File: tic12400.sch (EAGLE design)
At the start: 14 parts, among them X1 22-23-2031

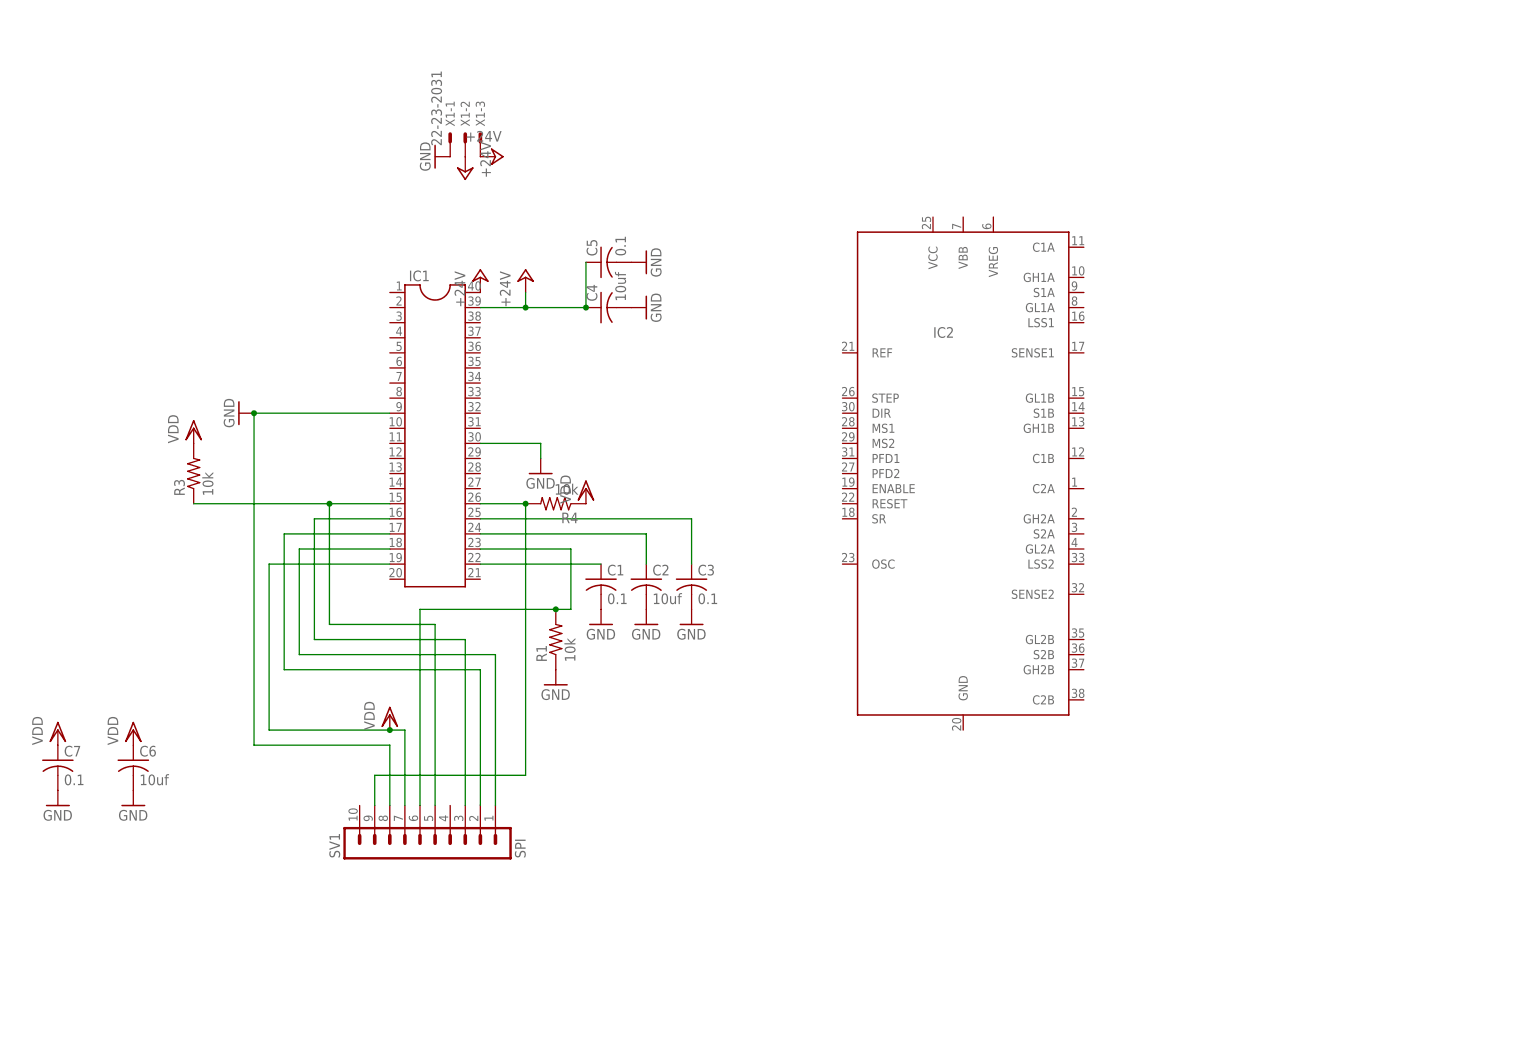
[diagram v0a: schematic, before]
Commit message: up
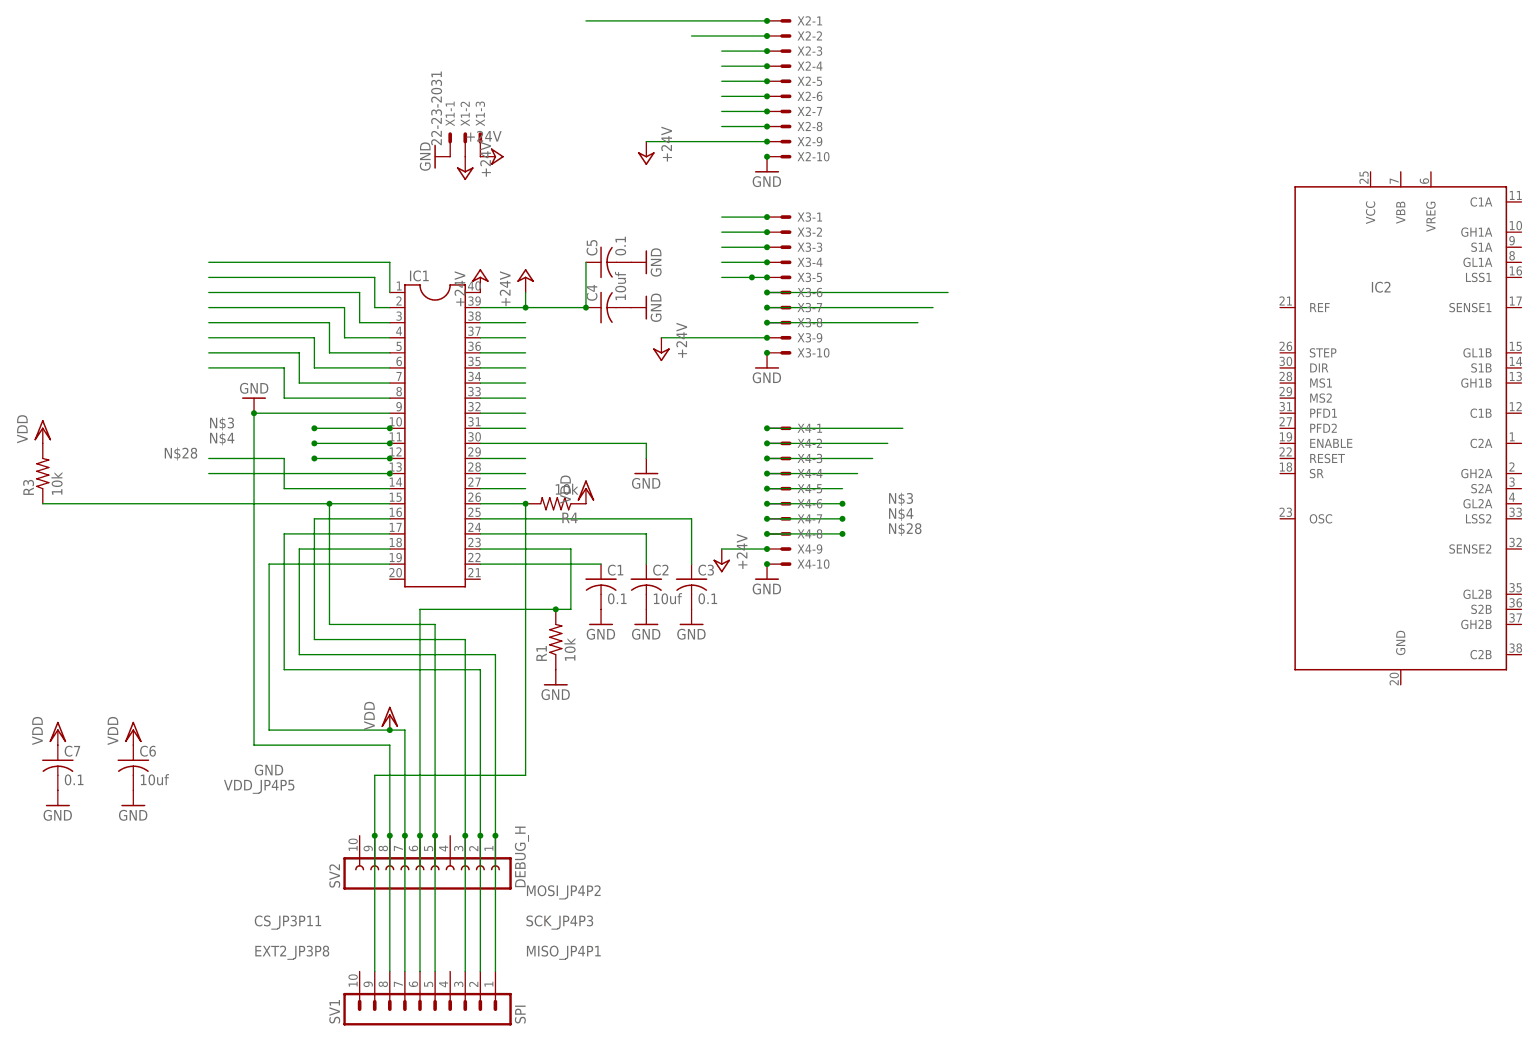
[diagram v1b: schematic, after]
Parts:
- added SV2: DEBUG_H, con-lsta:FE10-1
- added X2, X3, X4: (no value), con-molex:KK-156-10
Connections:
- removed net VDD: C6.1, C7.1, IC1.19, R3.2, R4.1, SV1.7
- new net CS_JP3P11: IC1.15, R3.1, SV1.5, SV2.5
- new net EXT2_JP3P8: IC1.26, R4.2, SV1.9, SV2.9
- new net GND_JP4P8: C1.2, C2.2, C3.2, C4.2, C5.2, C6.2, C7.2, IC1.30, R1.1, X1-1.S
- new net MISO_JP4P1: IC1.18, SV1.1, SV2.1
- new net MOSI_JP4P2: IC1.16, SV1.3, SV2.3
- new net N$1: IC1.13, X2-1.S
- new net N$11: IC1.6, X4-3.S
- new net N$12: IC1.5, X4-2.S
- new net N$13: IC1.4, X4-1.S
- new net N$14: IC1.3, X3-8.S
- new net N$15: IC1.2, X3-7.S
- new net N$16: IC1.1, X3-6.S
- new net N$17: IC1.27, X2-3.S
- new net N$18: IC1.28, X2-4.S
- new net N$19: IC1.29, X2-5.S
- new net N$20: IC1.31, X2-6.S
- new net N$21: IC1.32, X2-7.S
- new net N$22: IC1.33, X2-8.S
- new net N$23: IC1.34, X3-1.S
- new net N$24: IC1.35, X3-2.S
- new net N$25: IC1.36, X3-3.S
- new net N$26: IC1.37, X3-4.S
- new net N$27: IC1.38, X3-5.S
- new net N$28: IC1.12, X4-8.S
- new net SCK_JP4P3: IC1.17, SV1.2, SV2.2
- new net VDD_JP4P5: C6.1, C7.1, IC1.19, R3.2, R4.1, SV1.7, SV2.7
- net +24V: now also X2-9.S, X3-9.S, X4-9.S
- net GND: now also SV2.8, X2-10.S, X3-10.S, X4-10.S; no longer C1.2, C2.2, C3.2, C4.2, C5.2, C6.2, C7.2, IC1.30, R1.1, X1-1.S
- net N$2: now also IC1.14, X2-2.S; no longer IC1.18, SV1.1
- net N$3: now also IC1.10, X4-6.S; no longer IC1.16, SV1.3
- net N$4: now also IC1.11, X4-7.S; no longer IC1.17, SV1.2
- net N$5: now also IC1.8, X4-5.S; no longer IC1.15, R3.1, SV1.5
- net N$6: now also SV2.6
- net N$7: now also IC1.7, X4-4.S; no longer IC1.26, R4.2, SV1.9
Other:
- moved on the sheet: IC2, R3, SV1
